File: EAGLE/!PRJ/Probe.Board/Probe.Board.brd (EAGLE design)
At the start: 160 x 100 mm, 0 parts

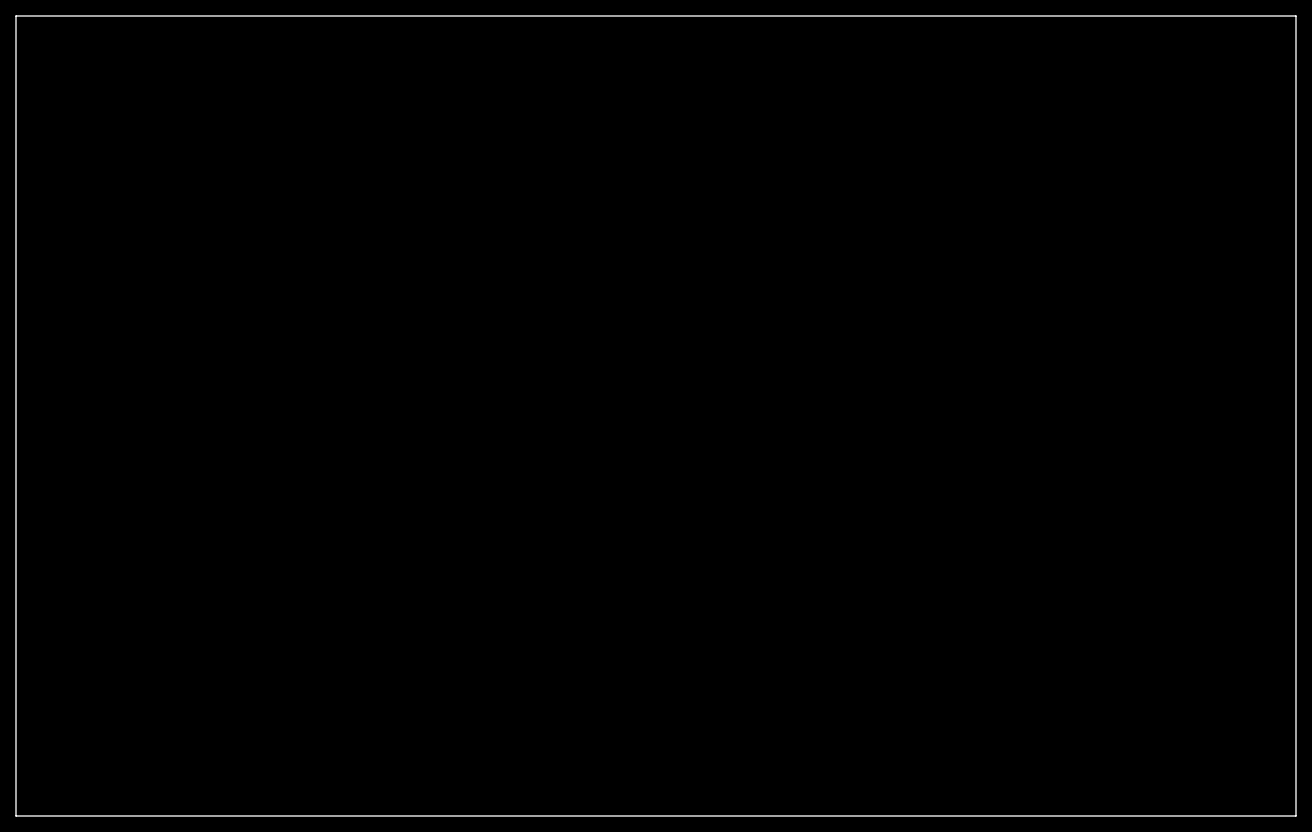
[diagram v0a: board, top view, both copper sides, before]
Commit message: 20180504
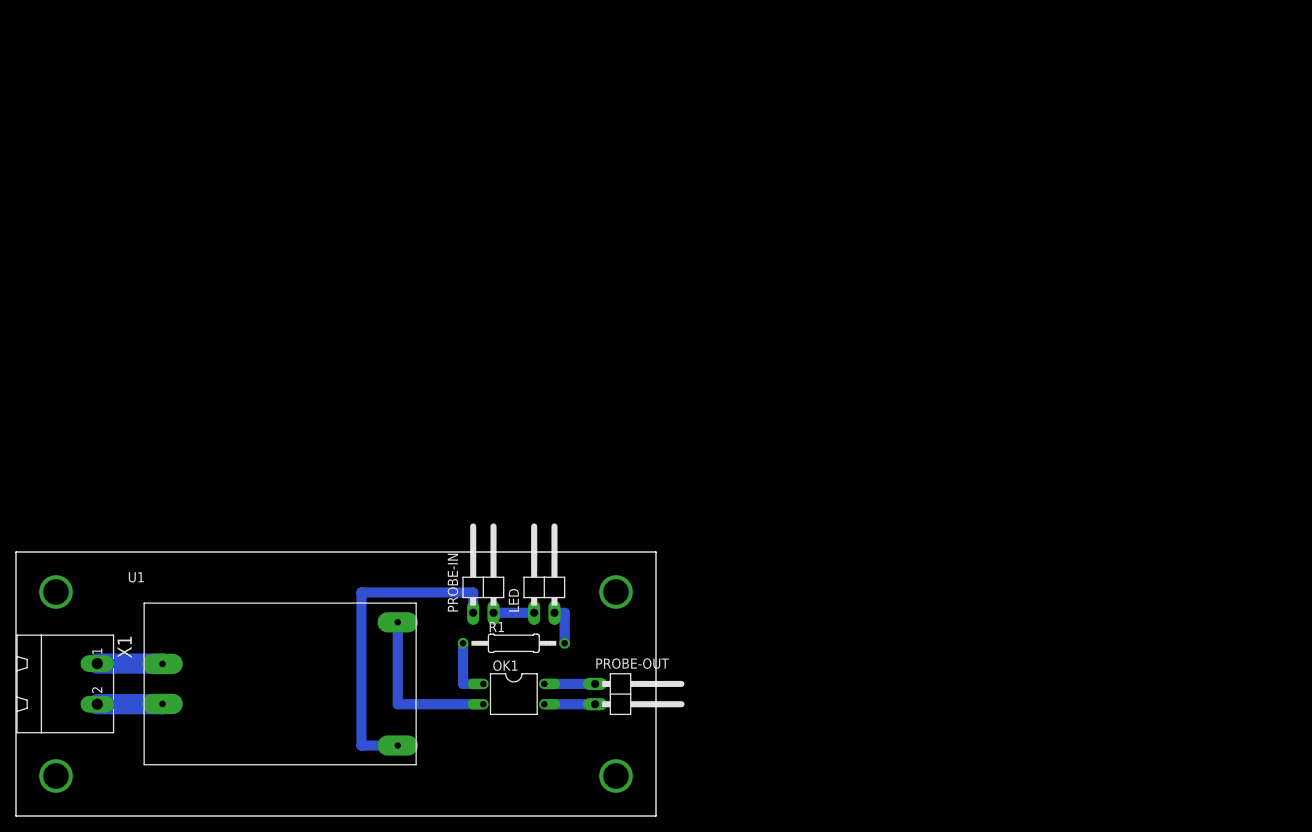
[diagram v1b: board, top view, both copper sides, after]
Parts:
- added LED, PROBE-IN, PROBE-OUT: (no value), pinhead:1X02/90
- added OK1: PC817, optocoupler:DIL04
- added R1: 100, rcl:0207/12
- added U1: TSP-05TSP-05, net173:TSP-05
- added X1: MSTBA2, con-phoenix-508:MSTBA2
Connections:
- new net GND: OK1.2, U1.P$3
- new net N$1: U1.P$2, X1.2
- new net N$2: U1.P$1, X1.1
- new net N$3: OK1.3, PROBE-OUT.2
- new net N$4: OK1.4, PROBE-OUT.1
- new net N$5: OK1.1, R1.1
- new net N$6: LED.2, R1.2
- new net N$7: LED.1, PROBE-IN.2
- new net N$8: PROBE-IN.1, U1.P$4
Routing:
- net N$8: track 0.00 -> 40.2 mm
- net GND: track 0.00 -> 20.9 mm
- net N$2: track 0.00 -> 8.20 mm
- net N$1: track 0.00 -> 8.20 mm
- net N$5: track 0.00 -> 7.62 mm
- net N$4: track 0.00 -> 6.35 mm
- net N$3: track 0.00 -> 6.35 mm
- net N$7: track 0.00 -> 5.08 mm
- net N$6: track 0.00 -> 5.08 mm
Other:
- board size 160 x 100 mm -> 80 x 33 mm
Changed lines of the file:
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@@
 <setting verticaltext="up"/>
 </settings>
-<grid distance="0.05" unitdist="inch" unit="inch" style="lines" multiple="1" display="no" altdistance="0.025" altunitdist="inch" altunit="inch"/>
+<grid distance="0.05" unitdist="inch" unit="inch" style="lines" multiple="1" display="yes" altdistance="0.025" altunitdist="inch" altunit="mm"/>
 <layers>
 <layer number="1" name="Top" color="4" fill="1" visible="yes" active="yes"/>
@@
 <board>
 <plain>
-<wire x1="0" y1="0" x2="160" y2="0" width="0" layer="20"/>
-<wire x1="160" y1="0" x2="160" y2="100" width="0" layer="20"/>
-<wire x1="160" y1="100" x2="0" y2="100" width="0" layer="20"/>
-<wire x1="0" y1="100" x2="0" y2="0" width="0" layer="20"/>
+<wire x1="0" y1="0" x2="80" y2="0" width="0" layer="20"/>
+<wire x1="80" y1="0" x2="80" y2="33" width="0" layer="20"/>
+<wire x1="80" y1="33" x2="0" y2="33" width="0" layer="20"/>
+<wire x1="0" y1="33" x2="0" y2="0" width="0" layer="20"/>
 </plain>
 <attributes>
@@
 </autorouter>
 <elements>
+<element name="PROBE-IN" library="pinhead" package="1X02/90" value="" x="58.42" y="29.21"/>
+<element name="PROBE-OUT" library="pinhead" package="1X02/90" value="" x="76.2" y="15.24" rot="R270"/>
+<element name="OK1" library="optocoupler" package="DIL04" value="PC817" x="62.23" y="15.24" rot="R270">
+<attribute name="OC_NEWARK" value="97K7059" x="62.23" y="15.24" size="1.778" layer="27" rot="R270" display="off"/>
+<attribute name="MPN" value="PC817X4J000F" x="62.23" y="15.24" size="1.778" layer="27" rot="R270" display="off"/>
+<attribute name="MF" value="" x="62.23" y="15.24" size="1.778" layer="27" rot="R270" display="off"/>
+<attribute name="OC_FARNELL" value="9707727" x="62.23" y="15.24" size="1.778" layer="27" rot="R270" display="off"/>
+</element>
+<element name="X1" library="con-phoenix-508" package="MSTBA2" value="MSTBA2" x="5.08" y="16.51" rot="R270"/>
+<element name="R1" library="rcl" package="0207/12" value="100" x="62.23" y="21.59"/>
+<element name="LED" library="pinhead" package="1X02/90" value="" x="66.04" y="29.21"/>
+<element name="U1" library="net173" package="TSP-05" value="TSP-05TSP-05" x="33.02" y="16.51"/>
 </elements>
 <signals>
+<signal name="GND">
+<contactref element="OK1" pad="2"/>
+<contactref element="U1" pad="P$3"/>
+<wire x1="47.72" y1="24.21" x2="47.72" y2="13.97" width="1.27" layer="16"/>
+<wire x1="47.72" y1="13.97" x2="58.42" y2="13.97" width="1.27" layer="16"/>
+</signal>
+<signal name="N$3">
+<contactref element="OK1" pad="3"/>
+<contactref element="PROBE-OUT" pad="2"/>
+<wire x1="66.04" y1="13.97" x2="72.39" y2="13.97" width="1.27" layer="16"/>
+</signal>
+<signal name="N$4">
+<contactref element="OK1" pad="4"/>
+<contactref element="PROBE-OUT" pad="1"/>
+<wire x1="66.04" y1="16.51" x2="72.39" y2="16.51" width="1.27" layer="16"/>
+</signal>
+<signal name="N$5">
+<contactref element="OK1" pad="1"/>
+<contactref element="R1" pad="1"/>
+<wire x1="58.42" y1="16.51" x2="55.88" y2="16.51" width="1.27" layer="16"/>
+<wire x1="55.88" y1="16.51" x2="55.88" y2="21.59" width="1.27" layer="16"/>
+</signal>
+<signal name="N$6">
+<contactref element="R1" pad="2"/>
+<contactref element="LED" pad="2"/>
+<wire x1="68.58" y1="21.59" x2="68.58" y2="25.4" width="1.27" layer="16"/>
+<wire x1="68.58" y1="25.4" x2="67.31" y2="25.4" width="1.27" layer="16"/>
+</signal>
+<signal name="N$7">
+<contactref element="LED" pad="1"/>
+<contactref element="PROBE-IN" pad="2"/>
+<wire x1="64.77" y1="25.4" x2="59.69" y2="25.4" width="1.27" layer="16"/>
+</signal>
+<signal name="N$8">
+<contactref element="PROBE-IN" pad="1"/>
+<contactref element="U1" pad="P$4"/>
+<wire x1="57.15" y1="25.4" x2="57.15" y2="27.94" width="1.27" layer="16"/>
+<wire x1="57.15" y1="27.94" x2="43.18" y2="27.94" width="1.27" layer="16"/>
+<wire x1="43.18" y1="27.94" x2="43.18" y2="8.81" width="1.27" layer="16"/>
+<wire x1="43.18" y1="8.81" x2="47.72" y2="8.81" width="1.27" layer="16"/>
+</signal>
+<signal name="N$9">
+<via x="5" y="5" extent="1-16" drill="3.2" shape="square"/>
+</signal>
+<signal name="N$10">
+<via x="5" y="28" extent="1-16" drill="3.2" shape="square"/>
+</signal>
+<signal name="N$11">
+<via x="75" y="28" extent="1-16" drill="3.2" shape="square"/>
+</signal>
+<signal name="N$12">
+<via x="75" y="5" extent="1-16" drill="3.2" shape="square"/>
+</signal>
+<signal name="N$1">
+<contactref element="X1" pad="2"/>
+<contactref element="U1" pad="P$2"/>
+<wire x1="10.16" y1="13.97" x2="18.32" y2="13.97" width="2.54" layer="16"/>
+<wire x1="18.32" y1="13.97" x2="18.32" y2="14.01" width="2.54" layer="16"/>
+</signal>
+<signal name="N$2">
+<contactref element="X1" pad="1"/>
+<contactref element="U1" pad="P$1"/>
+<wire x1="10.16" y1="19.05" x2="18.32" y2="19.05" width="2.54" layer="16"/>
+<wire x1="18.32" y1="19.05" x2="18.32" y2="19.01" width="2.54" layer="16"/>
+</signal>
 </signals>
 </board>
